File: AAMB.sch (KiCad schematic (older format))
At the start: 7 parts, among them J1 Screw_Terminal_01x04, J2 PJRAS4X2U01X, J3 SPKR L, J4 SPKR R, J5 Screw_Terminal_01x03, J6 Screw_Terminal_01x03, J7 Conn_01x04

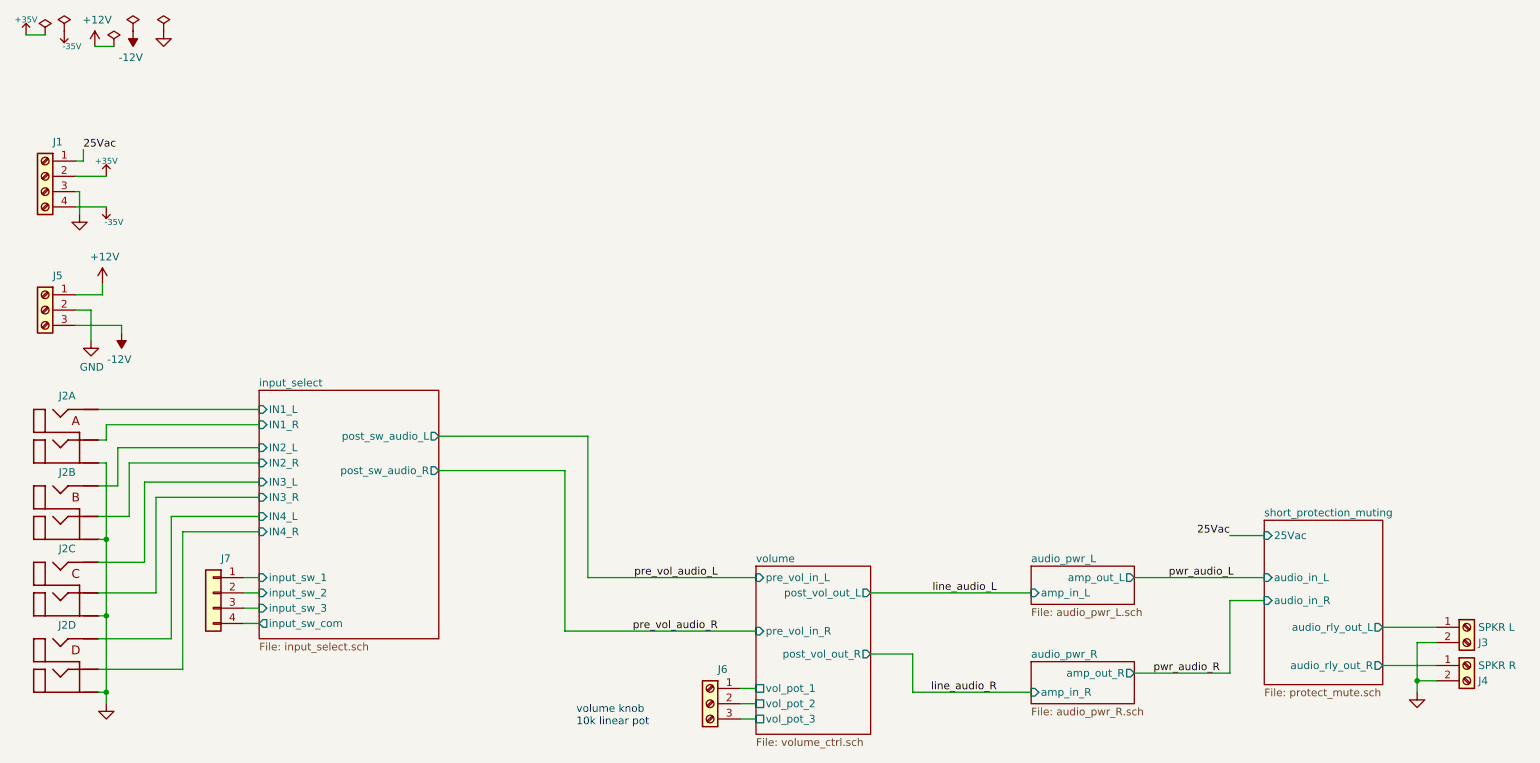
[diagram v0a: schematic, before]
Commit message: Schecmatic cleanup.
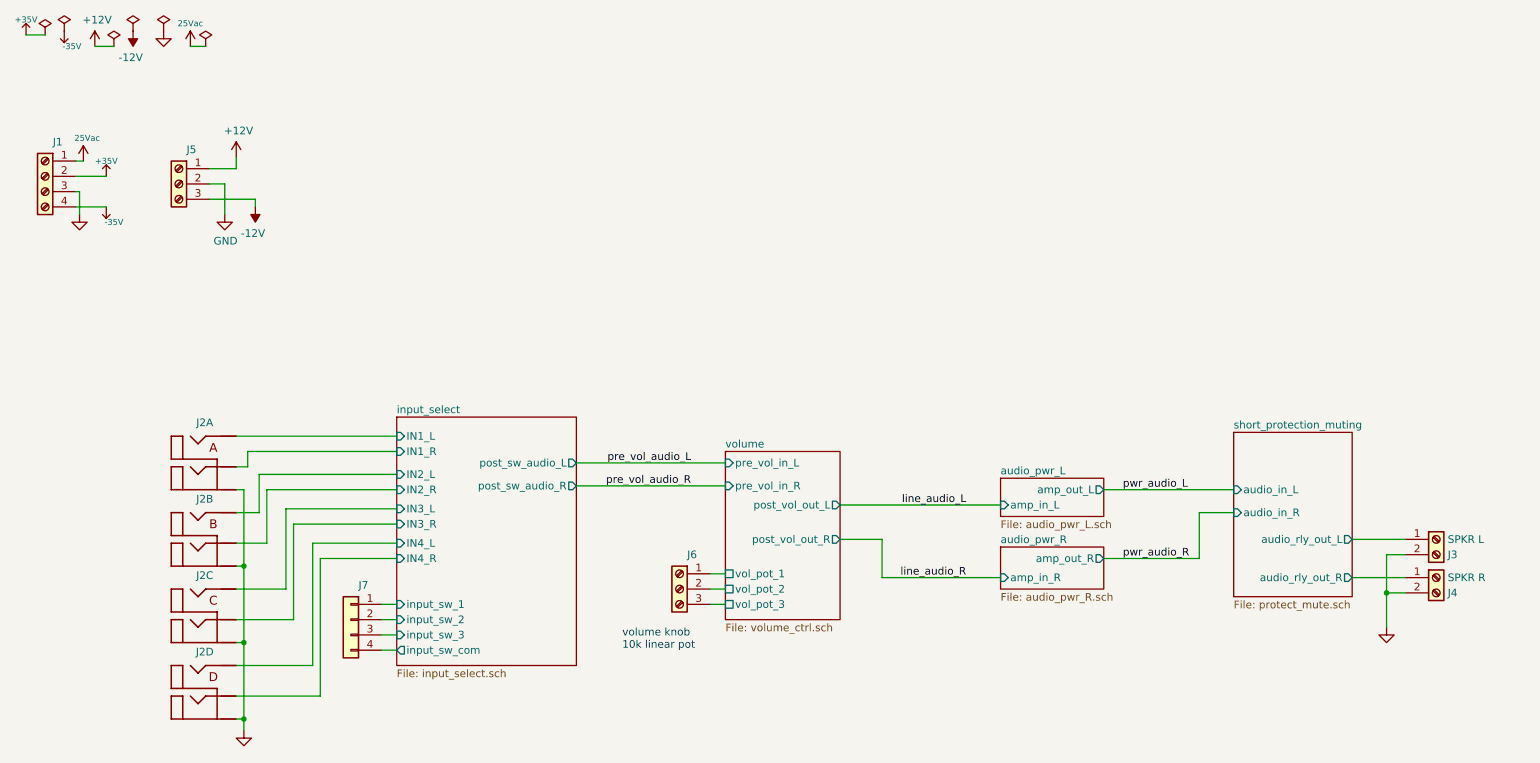
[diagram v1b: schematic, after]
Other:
- moved on the sheet: J2A, J2B, J2C, J2D, J3, J4, J5, J6, J7
